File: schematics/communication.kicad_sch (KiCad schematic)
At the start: 1 part

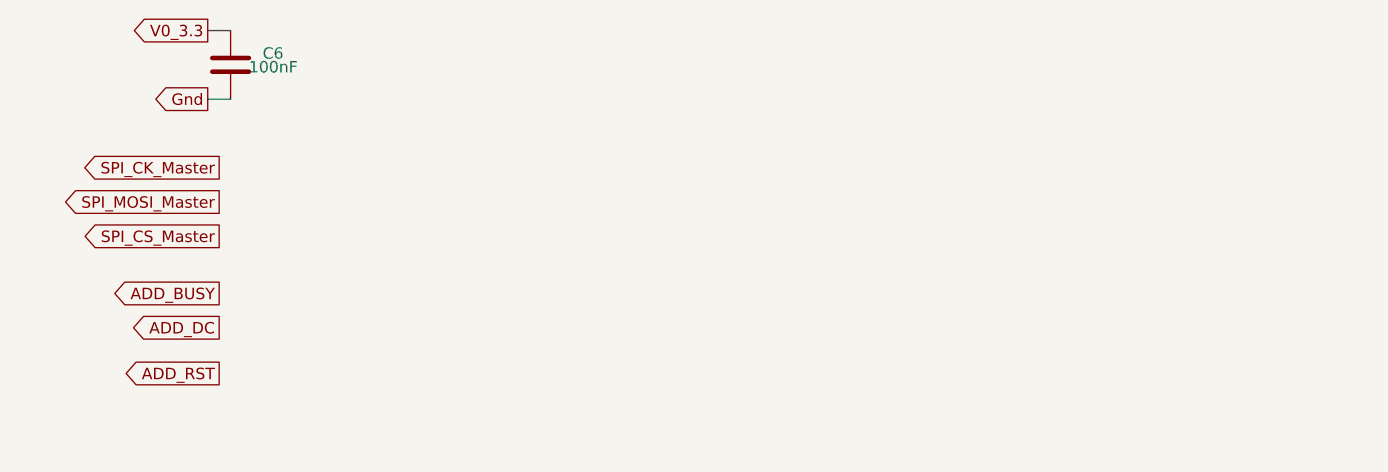
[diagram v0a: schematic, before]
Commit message: 2. | 2026-02-23 | Mo
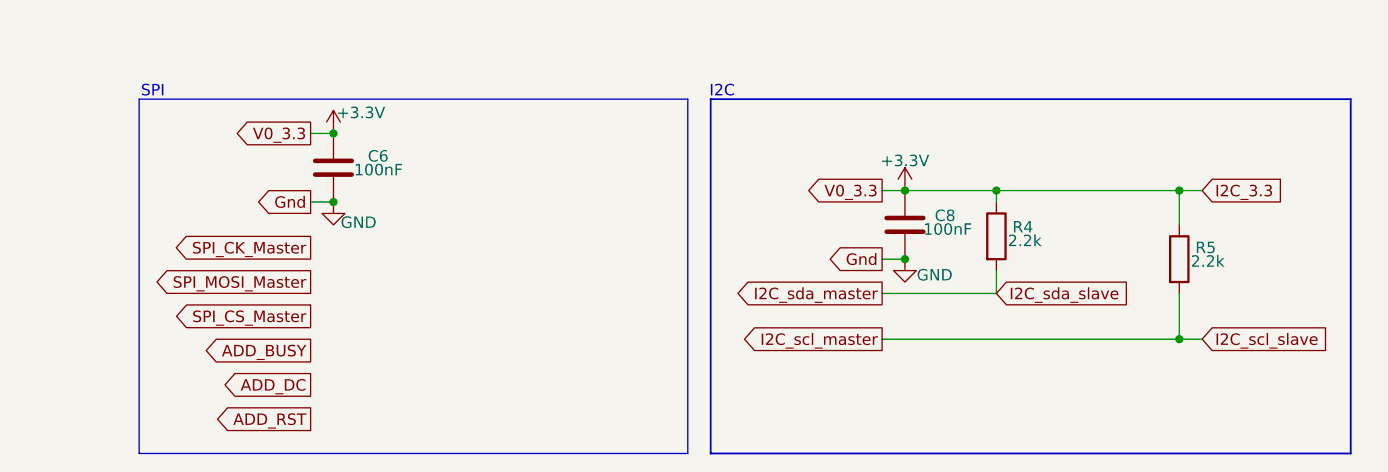
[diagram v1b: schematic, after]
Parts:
- added C8: 100nF, Capacitor_SMD:C_0603_1608Metric, symbol Device:C
- added R4, R5: 2.2k, Resistor_SMD:R_0402_1005Metric, symbol Device:R
- C6: footprint (none) -> Capacitor_SMD:C_0603_1608Metric
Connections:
- net Gnd renamed GND
- net GND: now also C8.2
- net V0_3.3 renamed +3.3V
- net +3.3V: now also C8.1, R4.1, R5.1
- new net I2C_scl_master: R5.2
- new net I2C_sda_master: R4.2
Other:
- note added: "I2C"
- note added: "SPI"
- moved on the sheet: C6

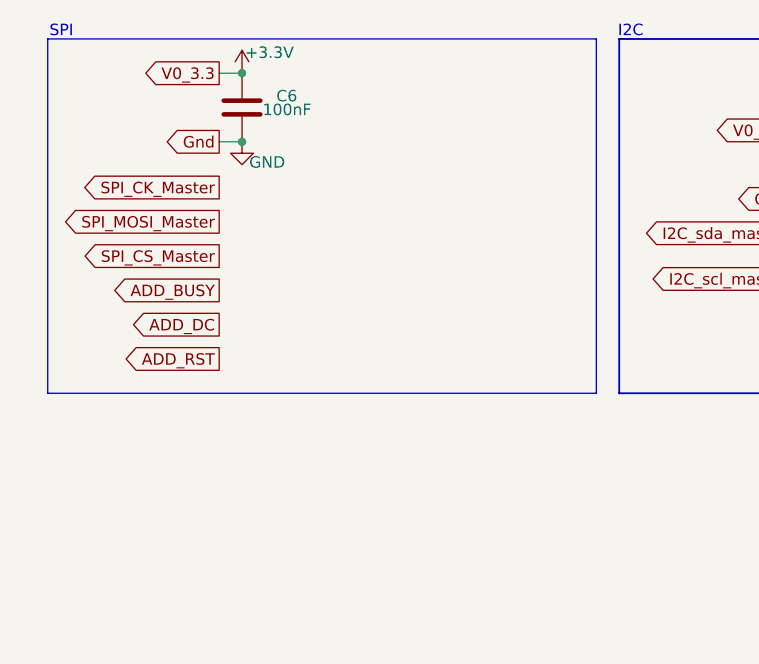
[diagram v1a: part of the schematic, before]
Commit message: 2026-02-25 | Mi
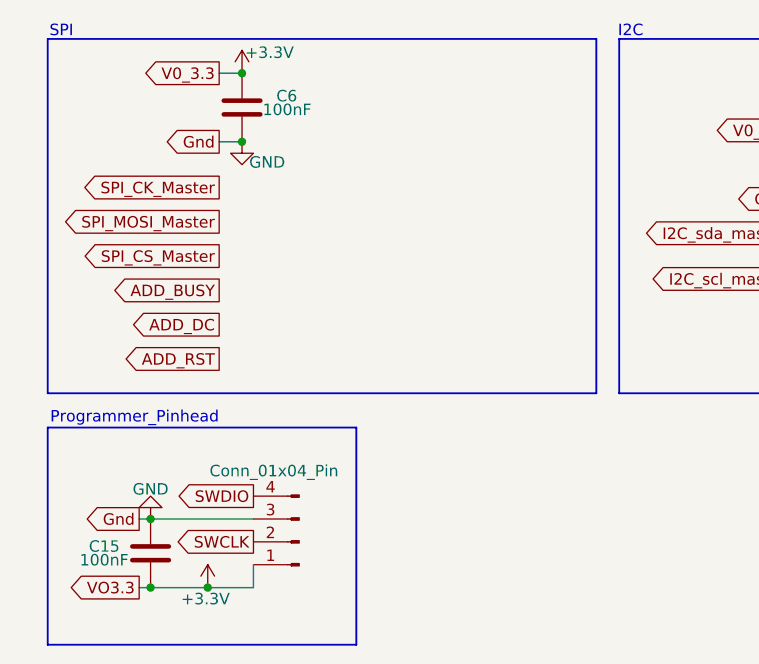
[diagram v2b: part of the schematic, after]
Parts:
- added C15: 100nF, Capacitor_SMD:C_0805_2012Metric, symbol Device:C
- added J2: Conn_01x04_Pin, Connector_PinHeader_1.00mm:PinHeader_1x04_P1.00mm_Vertical, symbol Connector:Conn_01x04_Pin
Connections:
- net +3.3V: now also C15.2, J2.1 (Pin_1)
- net GND: now also C15.1, J2.3 (Pin_3)
- new net SWCLK: J2.2 (Pin_2)
- new net SWDIO: J2.4 (Pin_4)
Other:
- note added: "Programmer_Pinhead"

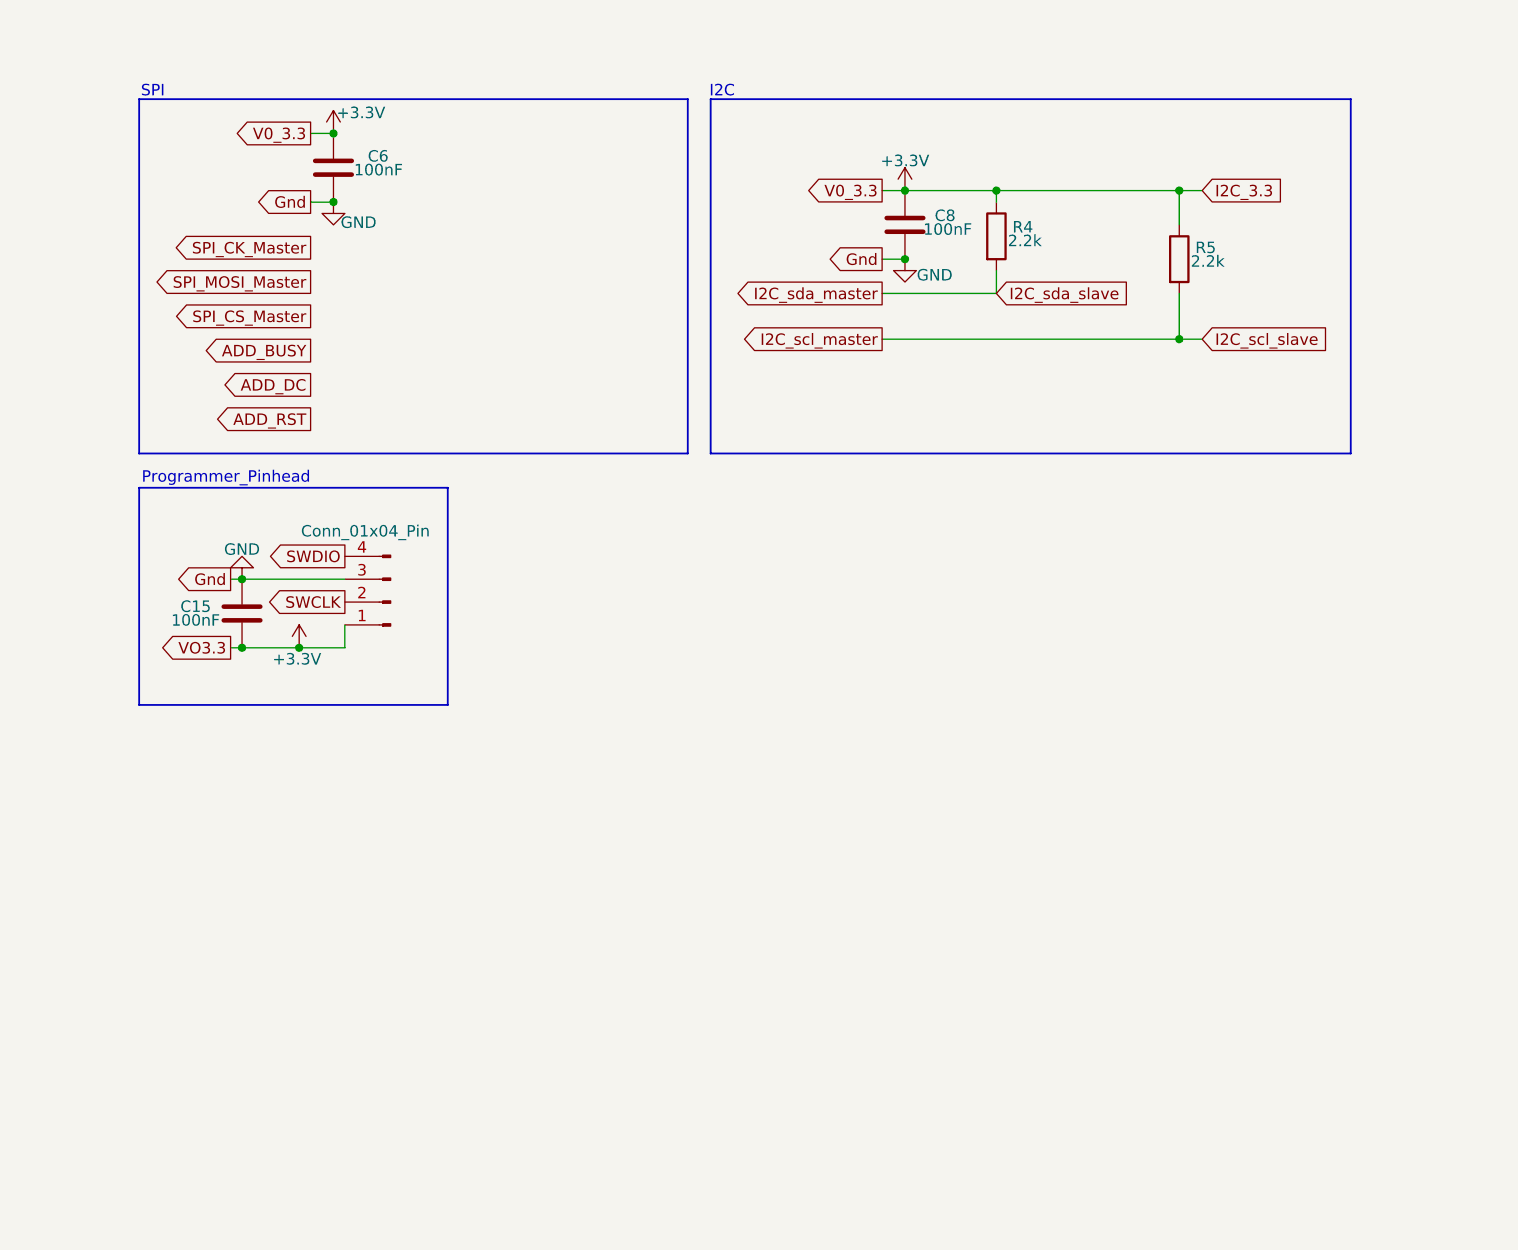
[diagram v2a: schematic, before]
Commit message: 2026-02-26 | Do
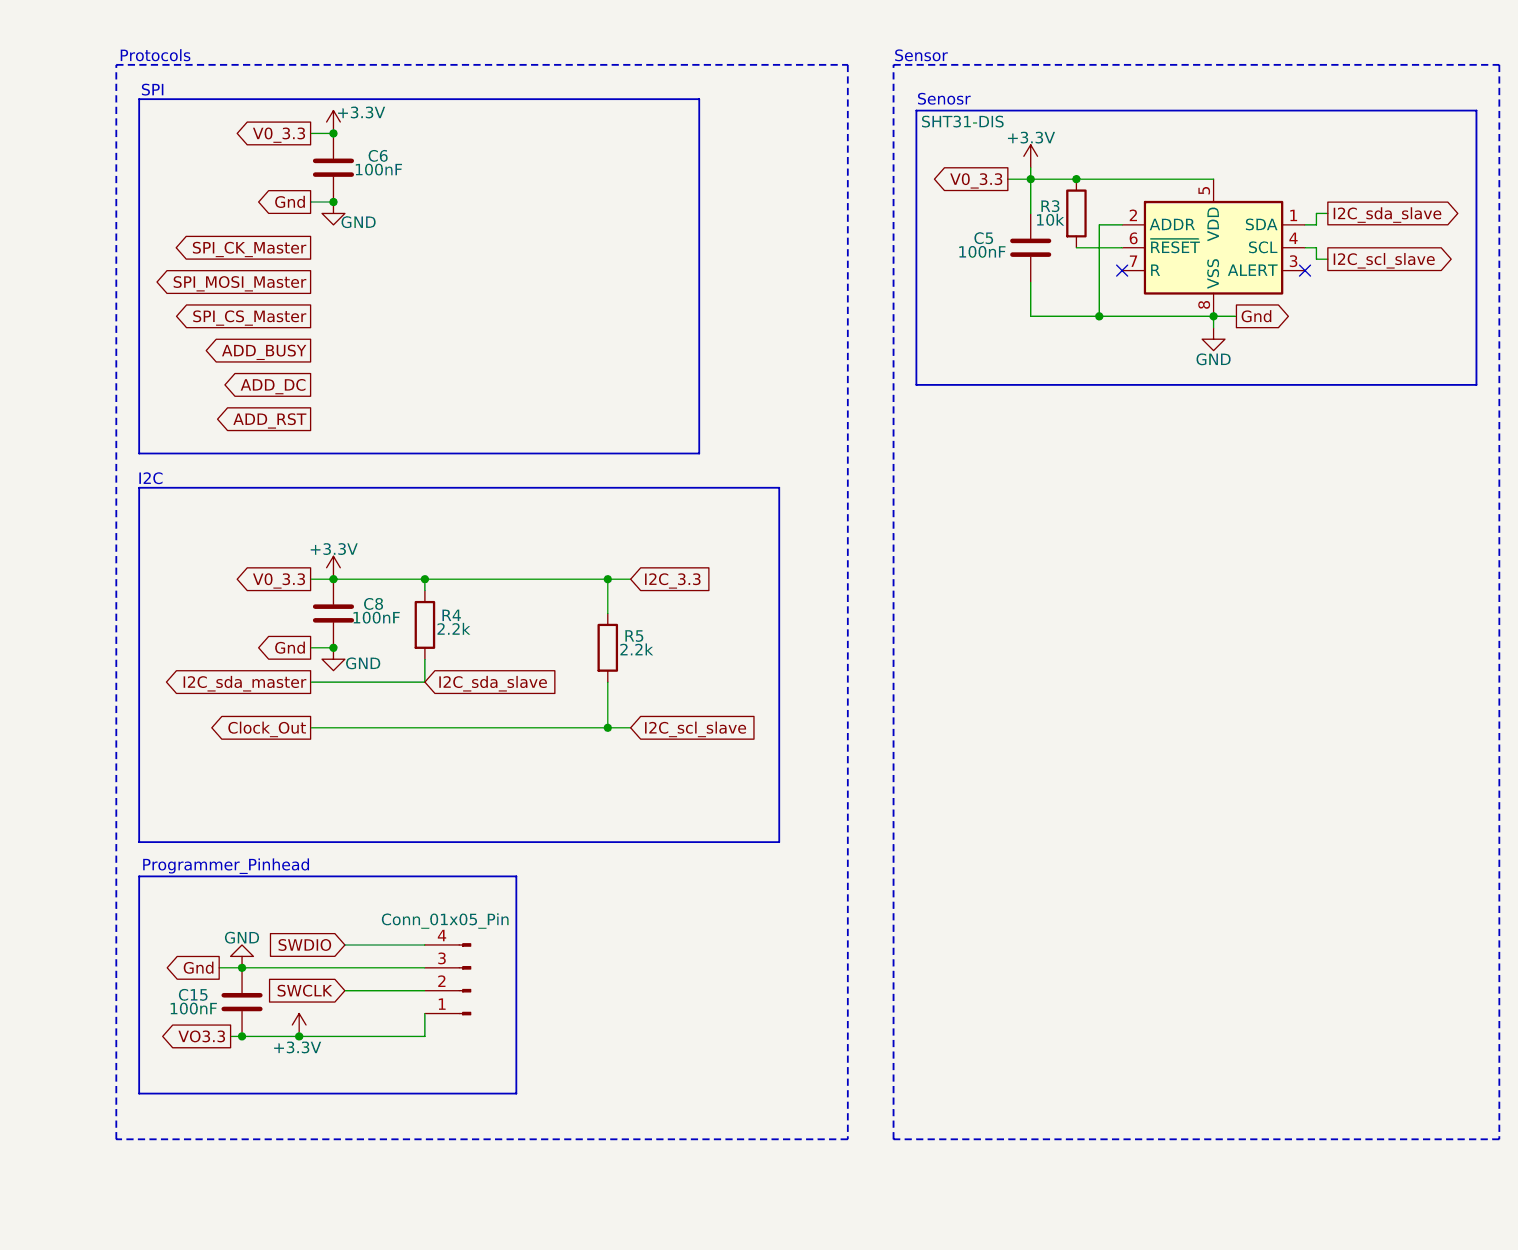
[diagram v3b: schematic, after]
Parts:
- added C5: 100nF, Capacitor_SMD:C_0603_1608Metric, symbol Device:C
- added R3: 10k, Resistor_SMD:R_0402_1005Metric, symbol Device:R
- added U3: SHT31-DIS, Sensor_Humidity:Texas_S-PWSON-N6-HDC2080, symbol Sensor_Humidity:SHT31-DIS
- C15: footprint Capacitor_SMD:C_0805_2012Metric -> Capacitor_SMD:C_0603_1608Metric
- J2: value Conn_01x04_Pin -> Conn_01x05_Pin
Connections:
- net +3.3V: now also C5.1, R3.1, U3.5 (VDD)
- net GND: now also C5.2, U3.2 (ADDR), U3.8 (VSS), U3.9 (VSS)
- net I2C_sda_master: now also U3.1 (SDA)
- net I2C_scl_master renamed Clock_Out
- net Clock_Out: now also U3.4 (SCL)
- new net: R3.2, U3.6 (~{RESET})
- no-connect marks 0 -> 2
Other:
- note added: "Protocols"
- note added: "Senosr"
- note added: "Sensor"
- title: Communication Protocols -> Additional stuff
- moved on the sheet: C15, C8, R4, R5

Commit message: 2026-02-28
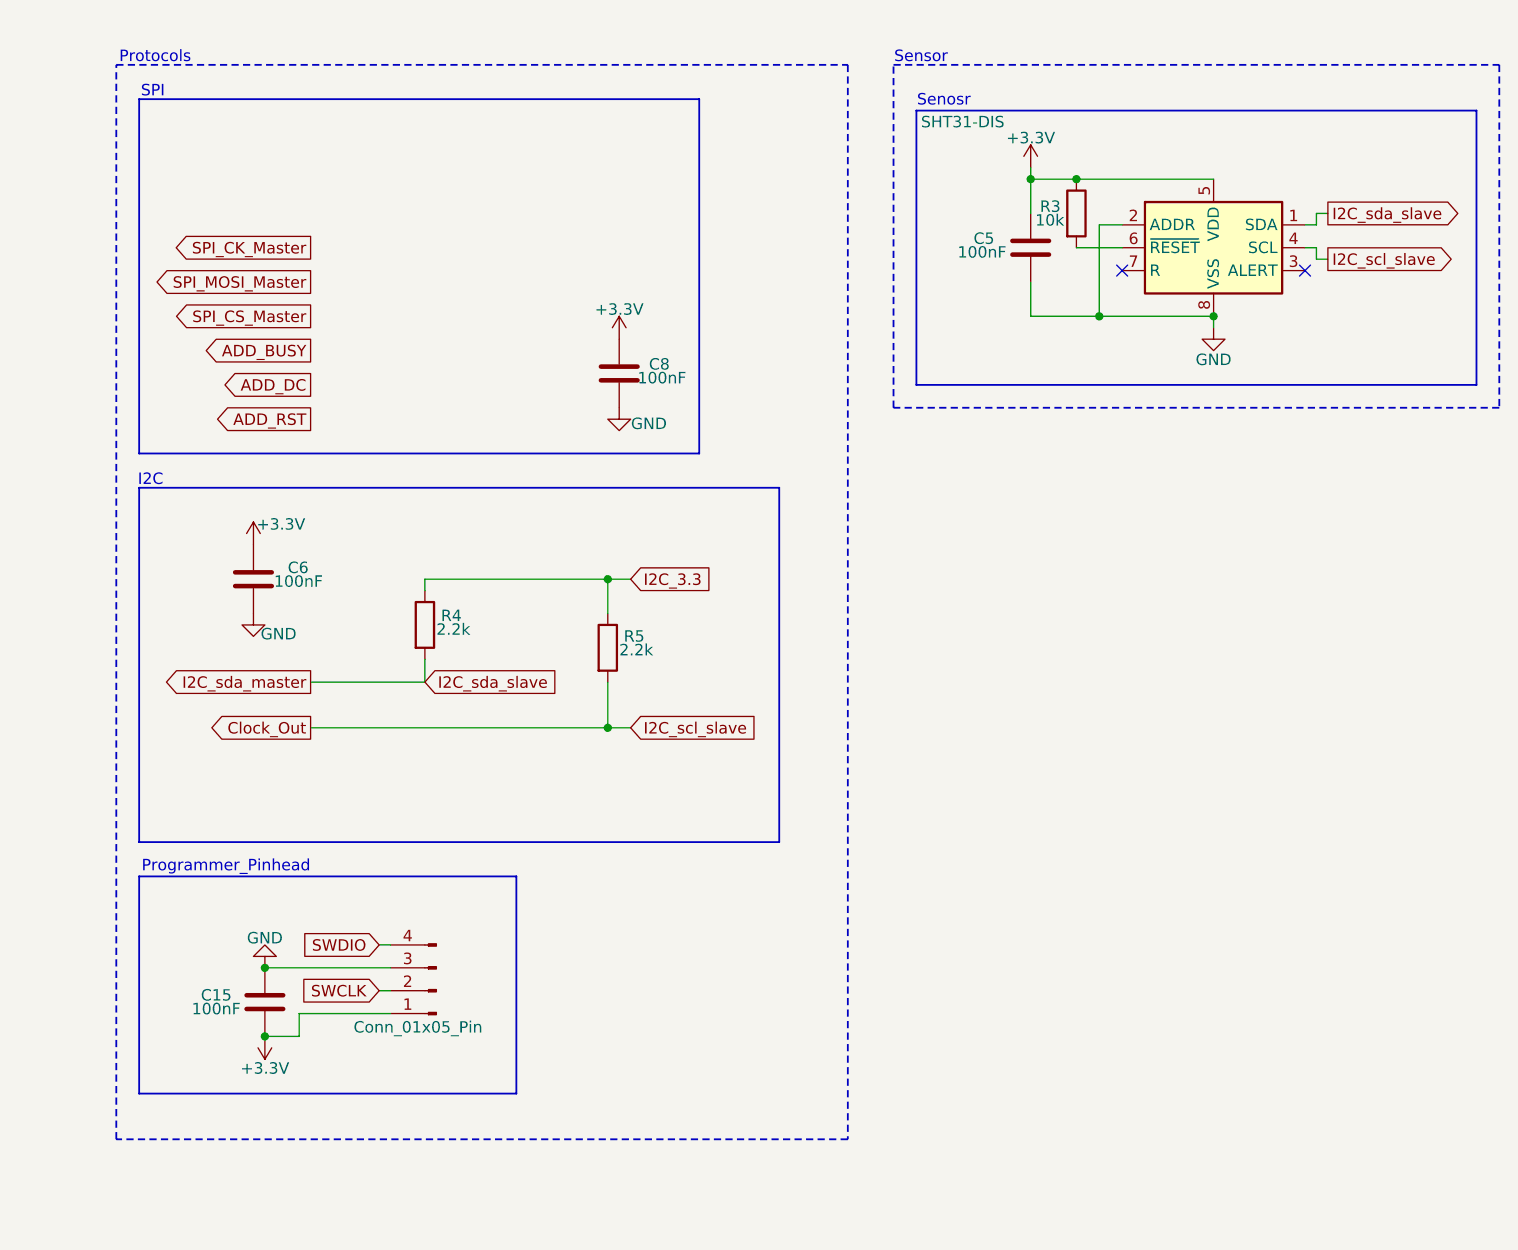
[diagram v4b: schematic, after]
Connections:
- net +3.3V: no longer R4.1, R5.1
- new net I2C_3.3: R4.1, R5.1
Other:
- moved on the sheet: C15, C6, C8
